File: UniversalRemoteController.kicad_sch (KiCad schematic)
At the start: 0 parts

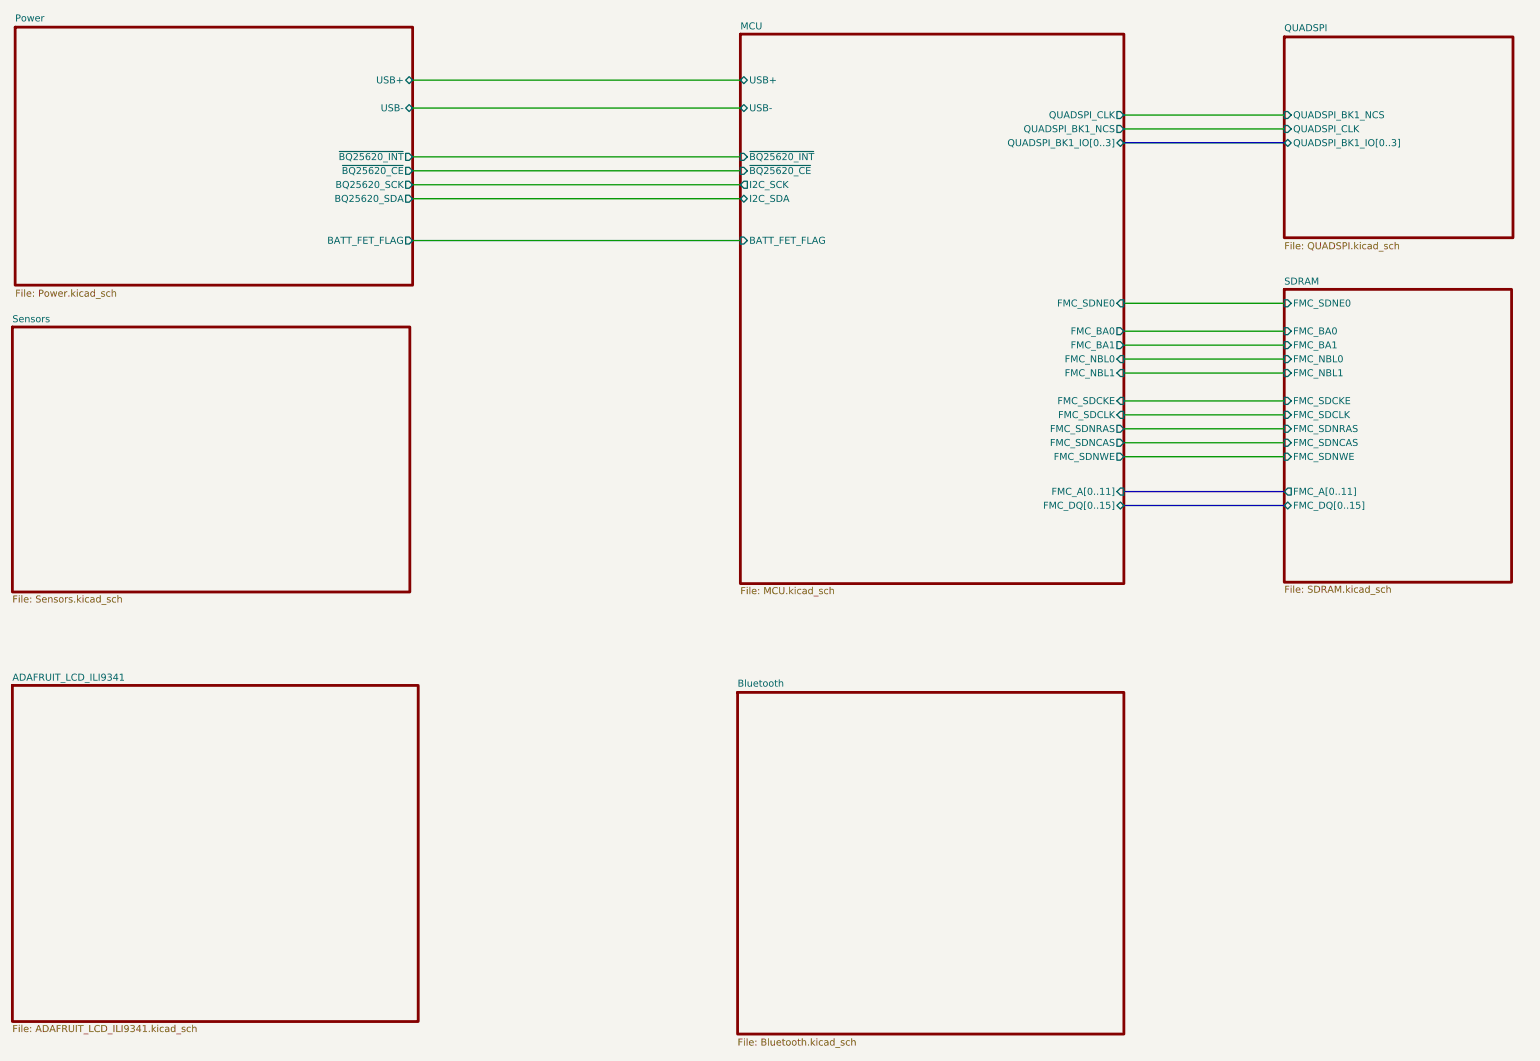
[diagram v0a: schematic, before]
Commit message: commit a sound version
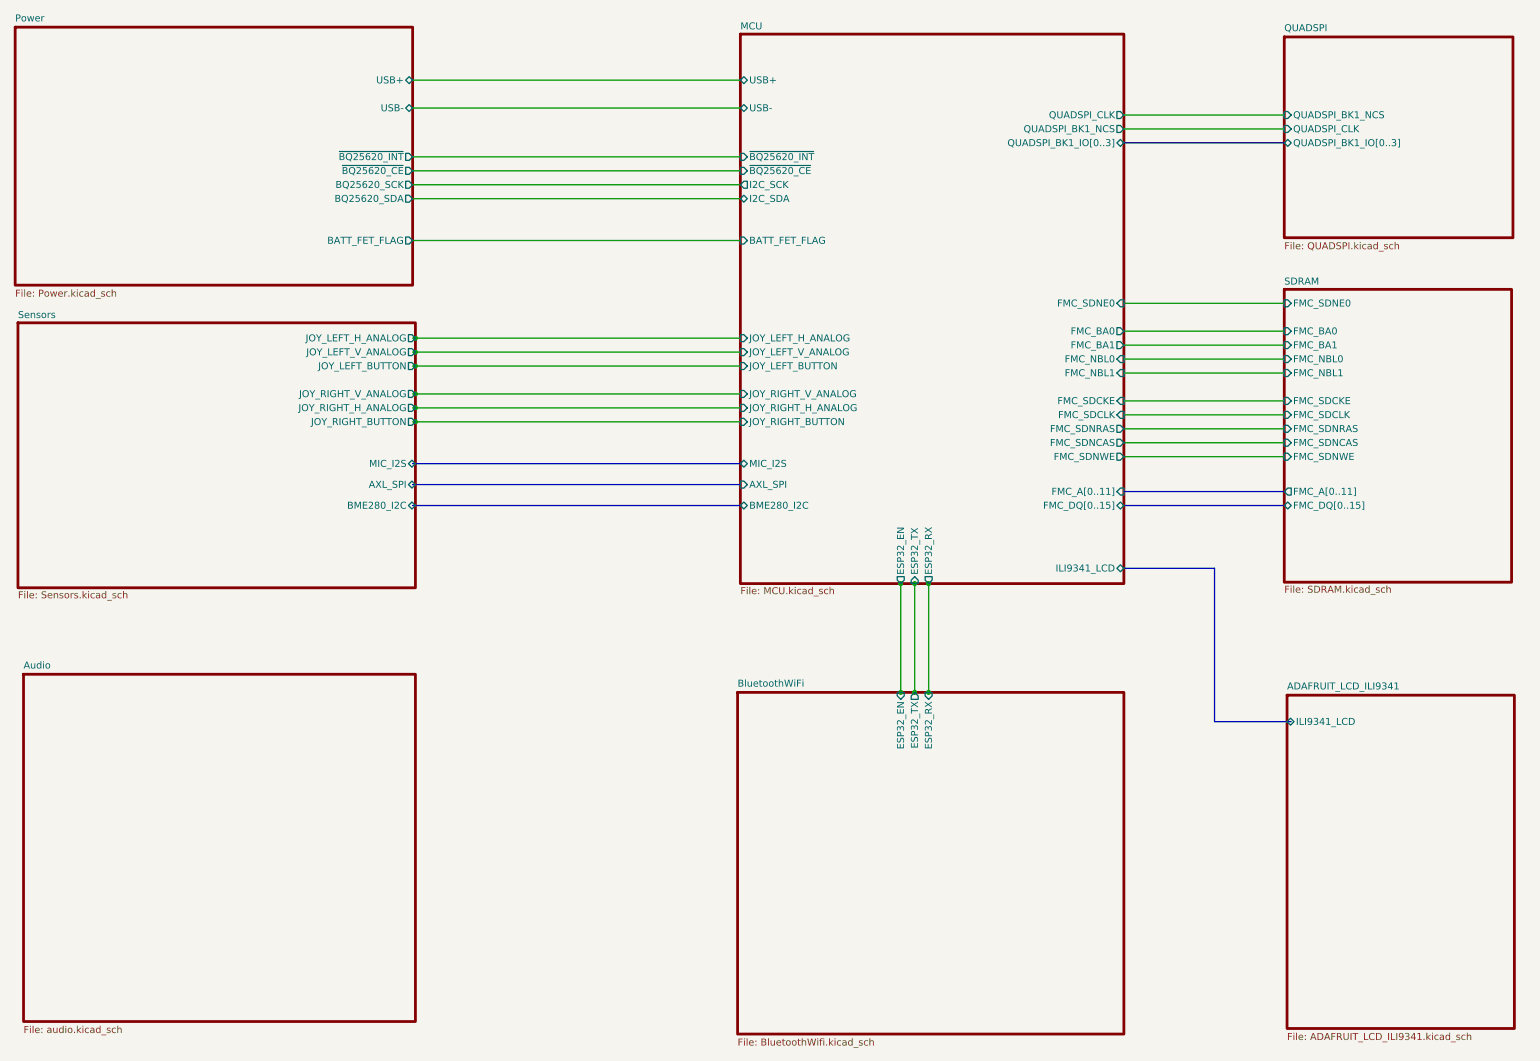
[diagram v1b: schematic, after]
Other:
- sheet Bluetooth renamed BluetoothWiFi
- added sheet Audio (audio.kicad_sch)
- sheet ADAFRUIT_LCD_ILI9341 ports: added ILI9341_LCD; removed none
- sheet BluetoothWiFi: file Bluetooth.kicad_sch -> BluetoothWifi.kicad_sch
- sheet BluetoothWiFi ports: added ESP32_EN, ESP32_RX, ESP32_TX; removed none
- sheet MCU ports: added AXL_SPI, BME280_I2C, ESP32_EN, ESP32_RX, ESP32_TX, ILI9341_LCD, JOY_LEFT_BUTTON, JOY_LEFT_H_ANALOG, JOY_LEFT_V_ANALOG, JOY_RIGHT_BUTTON, JOY_RIGHT_H_ANALOG, JOY_RIGHT_V_ANALOG, MIC_I2S; removed none
- sheet Sensors ports: added AXL_SPI, BME280_I2C, JOY_LEFT_BUTTON, JOY_LEFT_H_ANALOG, JOY_LEFT_V_ANALOG, JOY_RIGHT_BUTTON, JOY_RIGHT_H_ANALOG, JOY_RIGHT_V_ANALOG, MIC_I2S; removed none
